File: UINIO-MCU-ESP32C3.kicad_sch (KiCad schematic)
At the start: 43 parts, among them J1 Conn_01x15_Male, J2 外接串行下载接口, J3 Conn_01x15_Male, SW1 复位按键, SW2 下载按键, U1 ME6211C33M5G-N, U2 W25Q128JVSSIQ, U3 ESP32-C3, U4 CH343P, Y1 40MHz

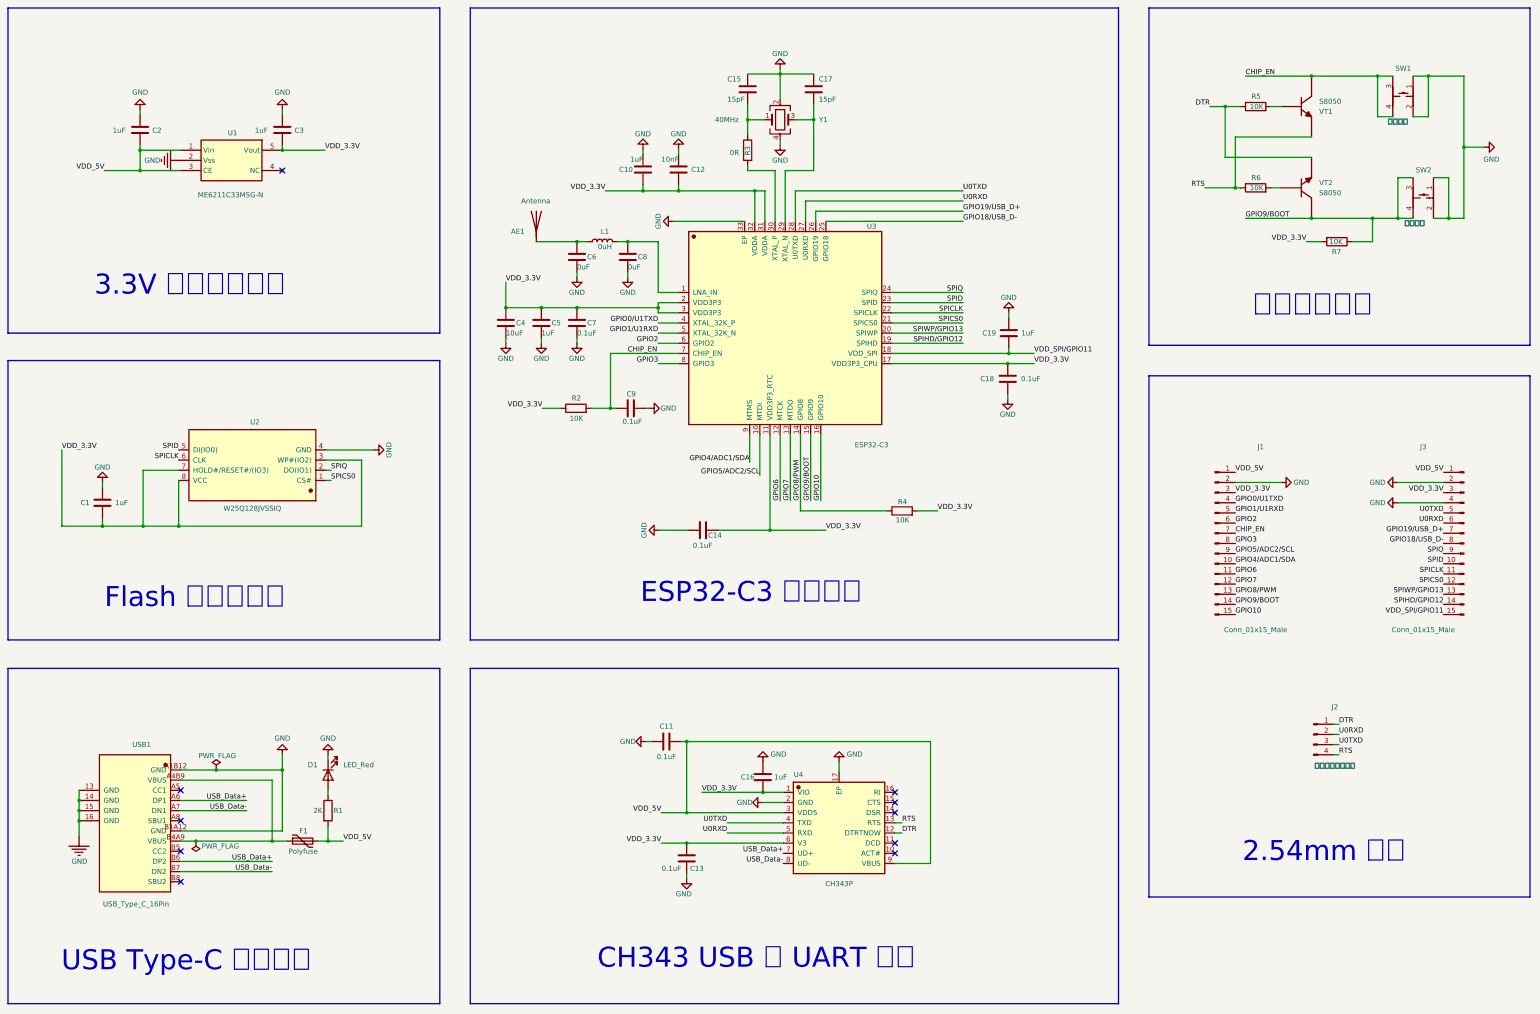
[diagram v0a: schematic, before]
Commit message: Finish PCB Layout.
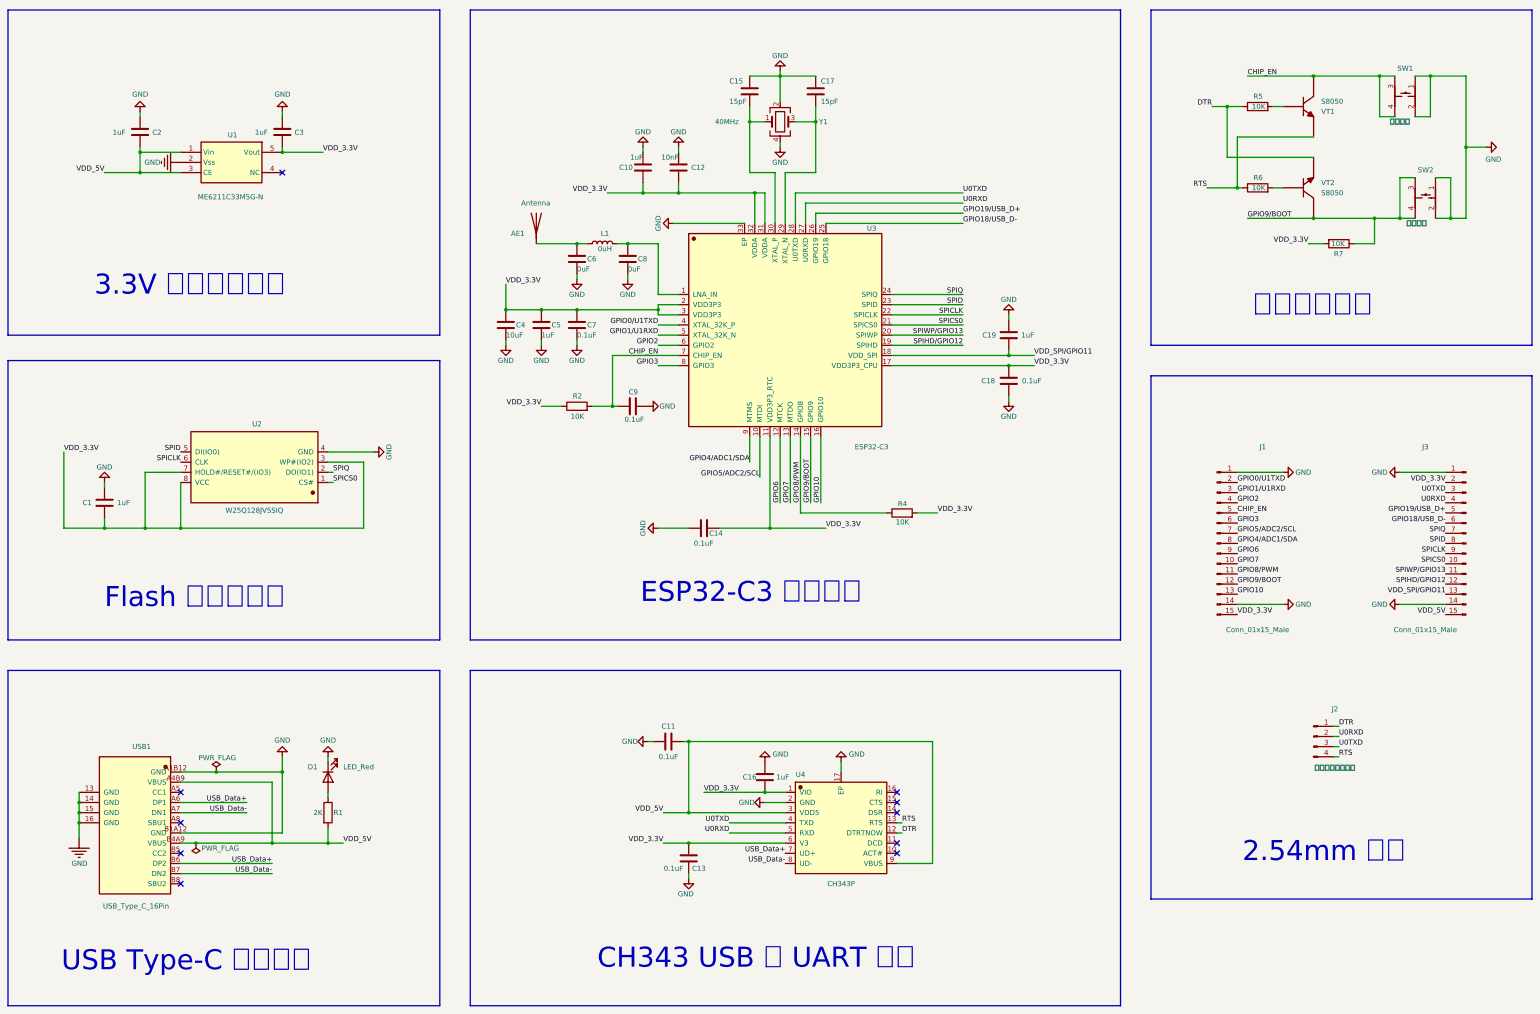
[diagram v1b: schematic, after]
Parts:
- removed F1: Polyfuse, Fuse:Fuse_1206_3216Metric, symbol Device:Polyfuse
- removed R3: 0R, Resistor_SMD:R_0402_1005Metric, symbol Device:R
- AE1: footprint RF_Antenna:Texas_SWRA117D_2.4GHz_Left -> RF_Antenna:Texas_SWRA117D_2.4GHz_Right
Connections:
- net CHIP_EN: now also J1.5 (Pin_5); no longer J1.7 (Pin_7)
- net GND: now also J1.1 (Pin_1), J1.14 (Pin_14), J3.1 (Pin_1), J3.14 (Pin_14); no longer J1.2 (Pin_2), J3.2 (Pin_2), J3.4 (Pin_4)
- net GPIO0/U1TXD: now also J1.2 (Pin_2); no longer J1.4 (Pin_4)
- net GPIO10: now also J1.13 (Pin_13); no longer J1.15 (Pin_15)
- net GPIO18/USB_D-: now also J3.6 (Pin_6); no longer J3.8 (Pin_8)
- net GPIO19/USB_D+: now also J3.5 (Pin_5); no longer J3.7 (Pin_7)
- net GPIO1/U1RXD: now also J1.3 (Pin_3); no longer J1.5 (Pin_5)
- net GPIO2: now also J1.4 (Pin_4); no longer J1.6 (Pin_6)
- net GPIO3: now also J1.6 (Pin_6); no longer J1.8 (Pin_8)
- net GPIO4/ADC1/SDA: now also J1.8 (Pin_8); no longer J1.10 (Pin_10)
- net GPIO5/ADC2/SCL: now also J1.7 (Pin_7); no longer J1.9 (Pin_9)
- net GPIO6: now also J1.9 (Pin_9); no longer J1.11 (Pin_11)
- net GPIO7: now also J1.10 (Pin_10); no longer J1.12 (Pin_12)
- net GPIO8/PWM: now also J1.11 (Pin_11); no longer J1.13 (Pin_13)
- net GPIO9/BOOT: now also J1.12 (Pin_12); no longer J1.14 (Pin_14)
- net SPICLK: now also J3.9 (Pin_9); no longer J3.11 (Pin_11)
- net SPICS0: now also J3.10 (Pin_10); no longer J3.12 (Pin_12)
- net SPID: now also J3.8 (Pin_8); no longer J3.10 (Pin_10)
- net SPIHD/GPIO12: now also J3.12 (Pin_12); no longer J3.14 (Pin_14)
- net SPIQ: now also J3.7 (Pin_7); no longer J3.9 (Pin_9)
- net SPIWP/GPIO13: now also J3.11 (Pin_11); no longer J3.13 (Pin_13)
- net U0RXD: now also J3.4 (Pin_4); no longer J3.6 (Pin_6)
- net U0TXD: now also J3.3 (Pin_3); no longer J3.5 (Pin_5)
- net VDD_3.3V: now also J1.15 (Pin_15), J3.2 (Pin_2); no longer J1.3 (Pin_3), J3.3 (Pin_3)
- net VDD_5V: now also J3.15 (Pin_15), USB1.A4B9 (VBUS), USB1.B4A9 (VBUS); no longer J1.1 (Pin_1), J3.1 (Pin_1)
- net VDD_SPI/GPIO11: now also J3.13 (Pin_13); no longer J3.15 (Pin_15)
- net at C15.2, Y1.1: now also U3.30 (XTAL_P)
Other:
- moved on the sheet: AE1, C1, C10, C11, C12, C13, C14, C15, C16, C17, C18, C19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
